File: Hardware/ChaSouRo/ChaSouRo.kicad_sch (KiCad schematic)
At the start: 38 parts, among them J3 Conn_ST_STDC14, U1 STM32G431CBUx, Y1 Crystal_GND24_Small

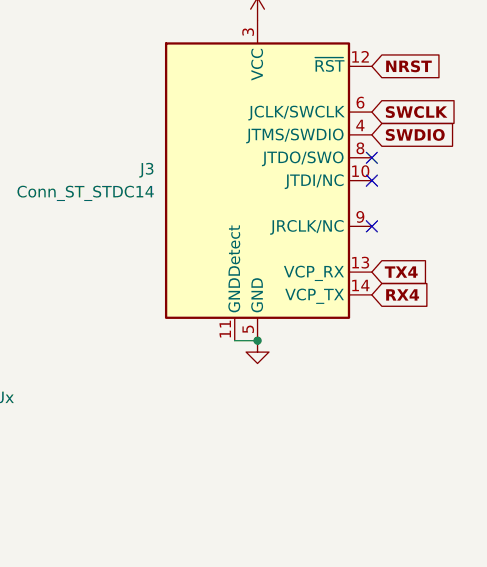
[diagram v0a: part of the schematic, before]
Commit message: check pcb LF
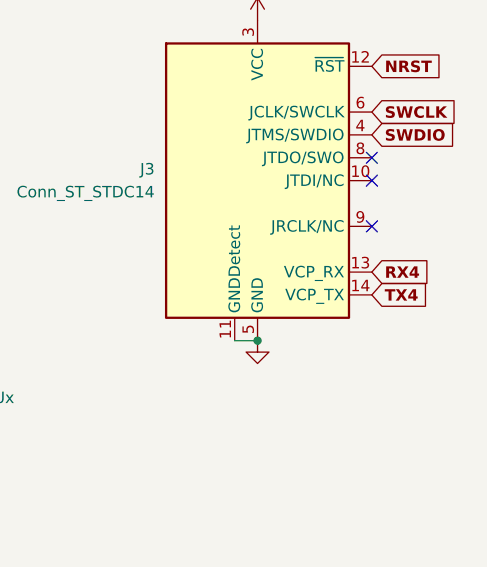
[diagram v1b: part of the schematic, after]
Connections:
- net RX4: now also J3.13 (VCP_RX); no longer J3.14 (VCP_TX)
- net TX4: now also J3.14 (VCP_TX); no longer J3.13 (VCP_RX)
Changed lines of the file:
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@@
 	(global_label "RX4"
 		(shape input)
-		(at 270.51 129.54 0)
+		(at 270.51 127 0)
 		(fields_autoplaced yes)
 		(effects
@@
 		)
 		(property "Intersheetrefs" "${INTERSHEET_REFS}"
-			(at 277.6602 129.54 0)
+			(at 277.6602 127 0)
 			(effects
 				(font
@@
 	(global_label "TX4"
 		(shape input)
-		(at 270.51 127 0)
+		(at 270.51 129.54 0)
 		(fields_autoplaced yes)
 		(effects
@@
 		)
 		(property "Intersheetrefs" "${INTERSHEET_REFS}"
-			(at 277.3578 127 0)
-			(effects
-				(font
+			(at 277.3578 129.54 0)
+			(effects
+				(font
